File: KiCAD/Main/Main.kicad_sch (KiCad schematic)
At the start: 2 parts, among them J7 Conn_02x05_Top_Bottom_Mountin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

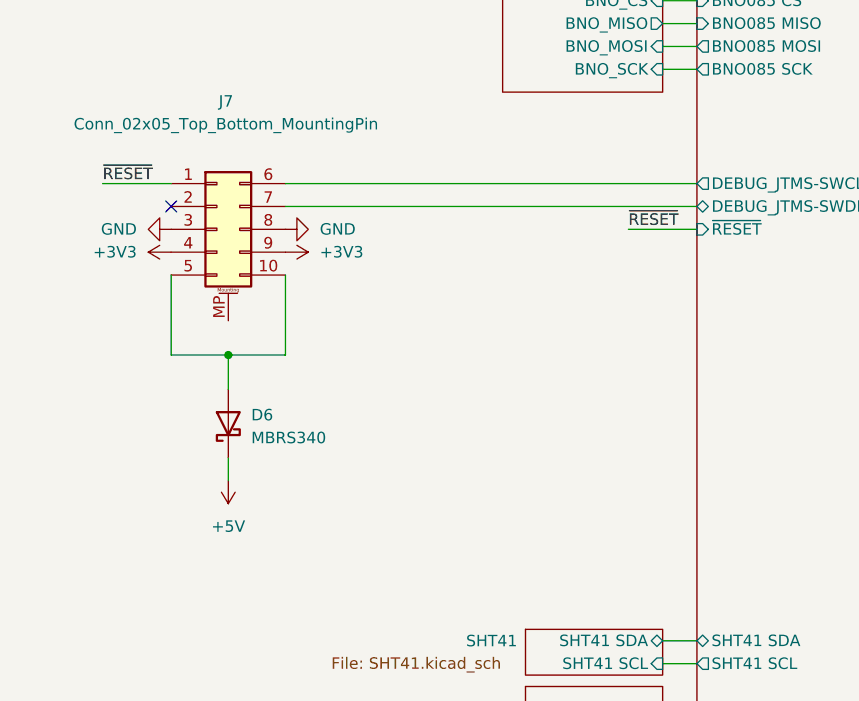
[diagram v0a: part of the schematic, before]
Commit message: Complete layout first draft
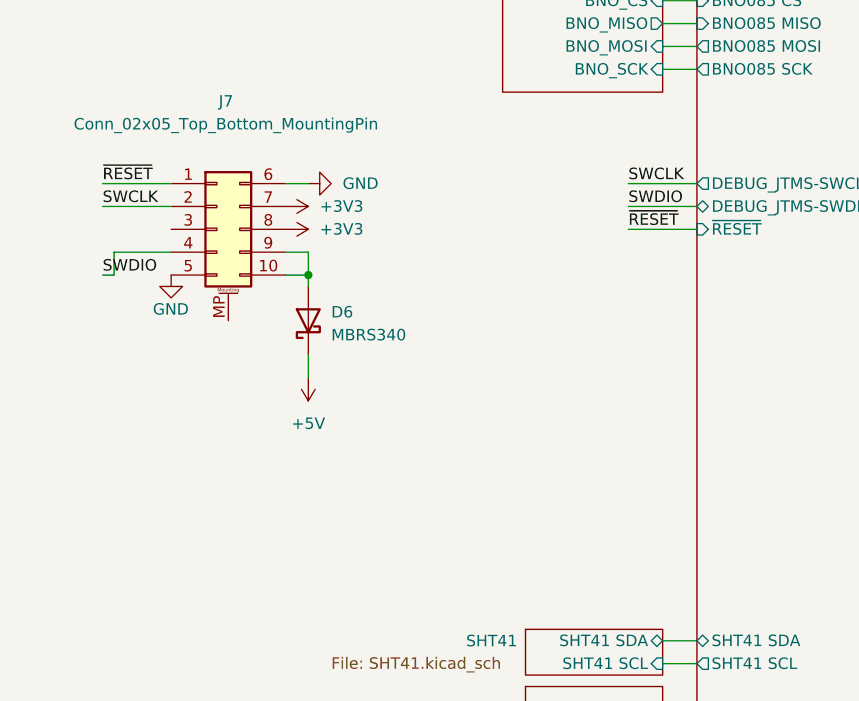
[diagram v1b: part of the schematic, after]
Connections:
- net Microcontroller/DEBUG_JTMS-SWCLK is gone; now on net GND: J7.6 (Pin_6)
- net Microcontroller/DEBUG_JTMS-SWDIO is gone; now on net +3V3: J7.7 (Pin_7)
- net +3V3: now also J7.8 (Pin_8); no longer J7.4 (Pin_4), J7.9 (Pin_9)
- net GND: now also J7.5 (Pin_5); no longer J7.3 (Pin_3), J7.8 (Pin_8)
- net at D6.2 (A), J7.10 (Pin_10): now also J7.9 (Pin_9); no longer J7.5 (Pin_5)
- net SWCLK: now reaches J7.2 (Pin_2)
- new net SWDIO: J7.4 (Pin_4)
- no-connect marks 1 -> 0
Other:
- moved on the sheet: D6
